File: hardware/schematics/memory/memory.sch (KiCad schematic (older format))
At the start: 5 parts

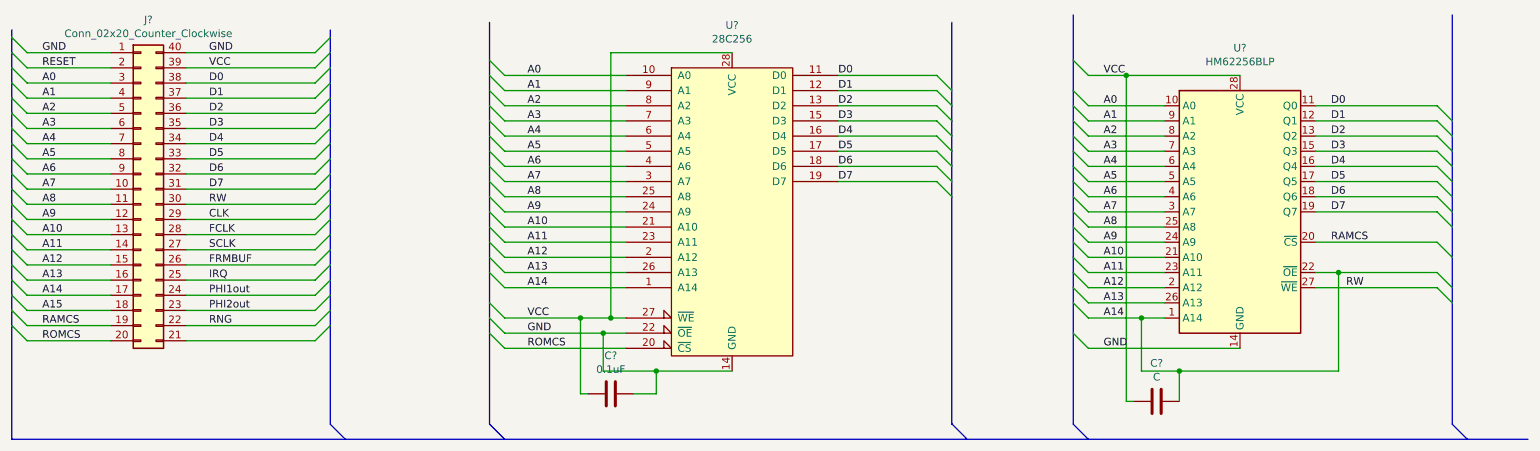
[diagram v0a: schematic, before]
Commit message: I started working on the PCBs
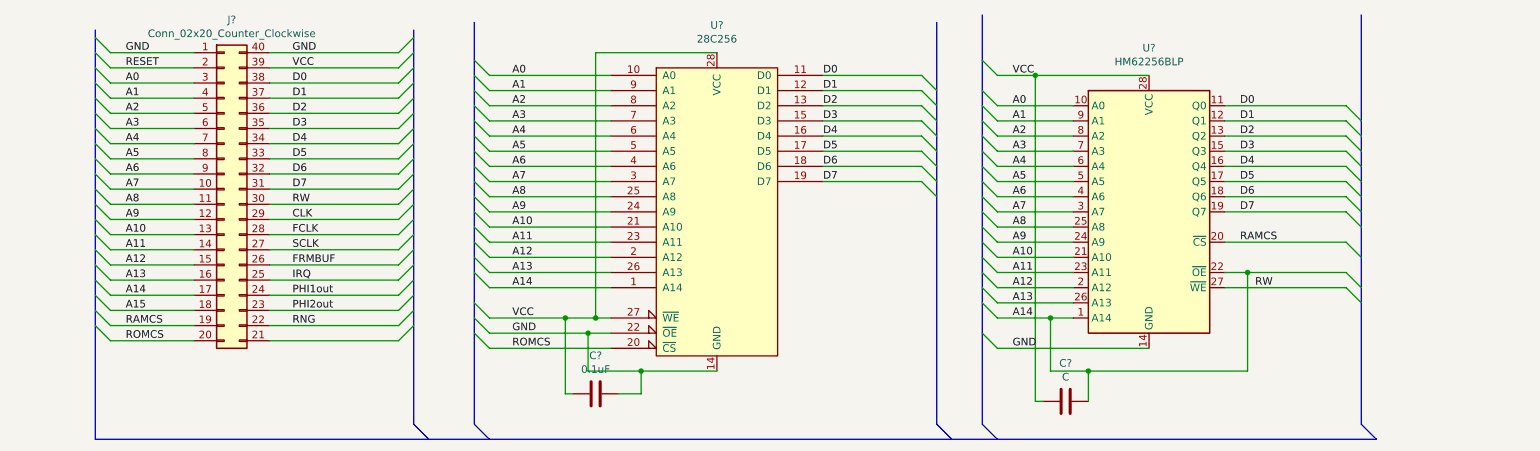
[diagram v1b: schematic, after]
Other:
- moved on the sheet: C?, J?, U?
